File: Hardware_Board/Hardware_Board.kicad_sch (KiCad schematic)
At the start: 0 parts

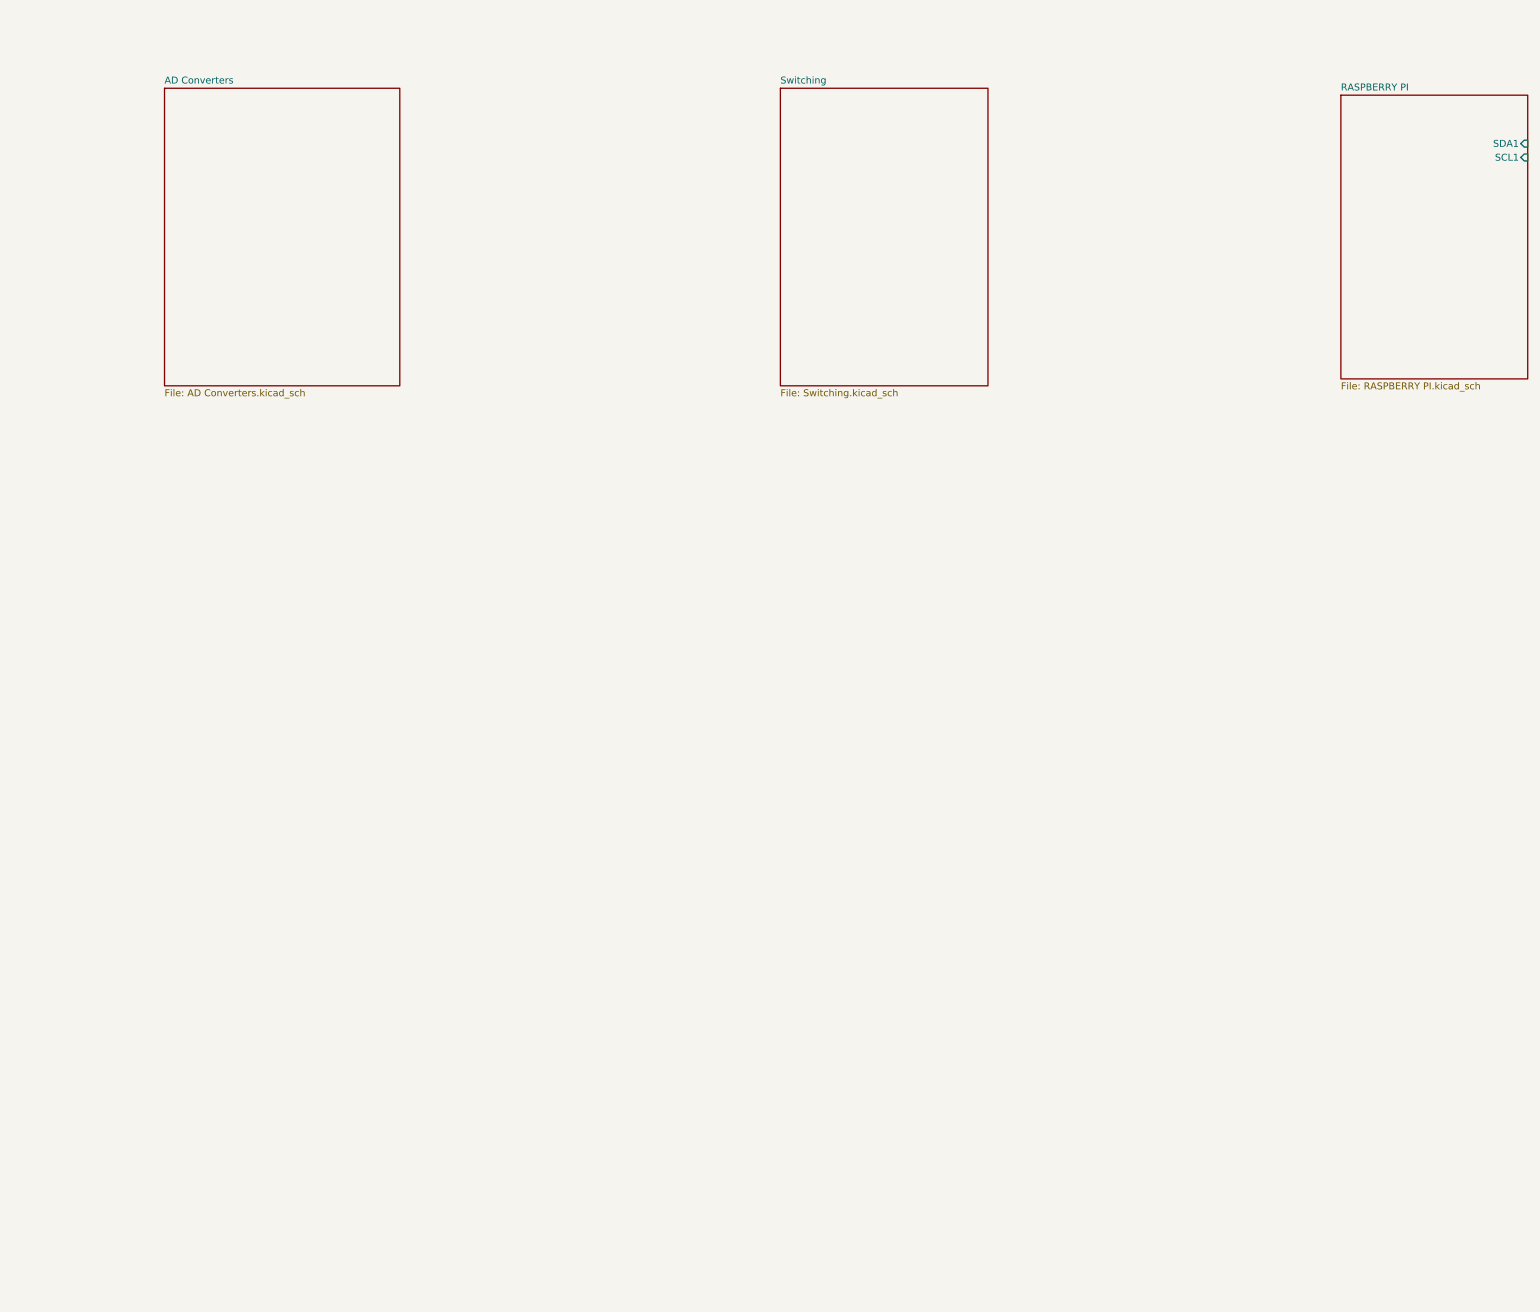
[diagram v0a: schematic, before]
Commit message: esc board updated
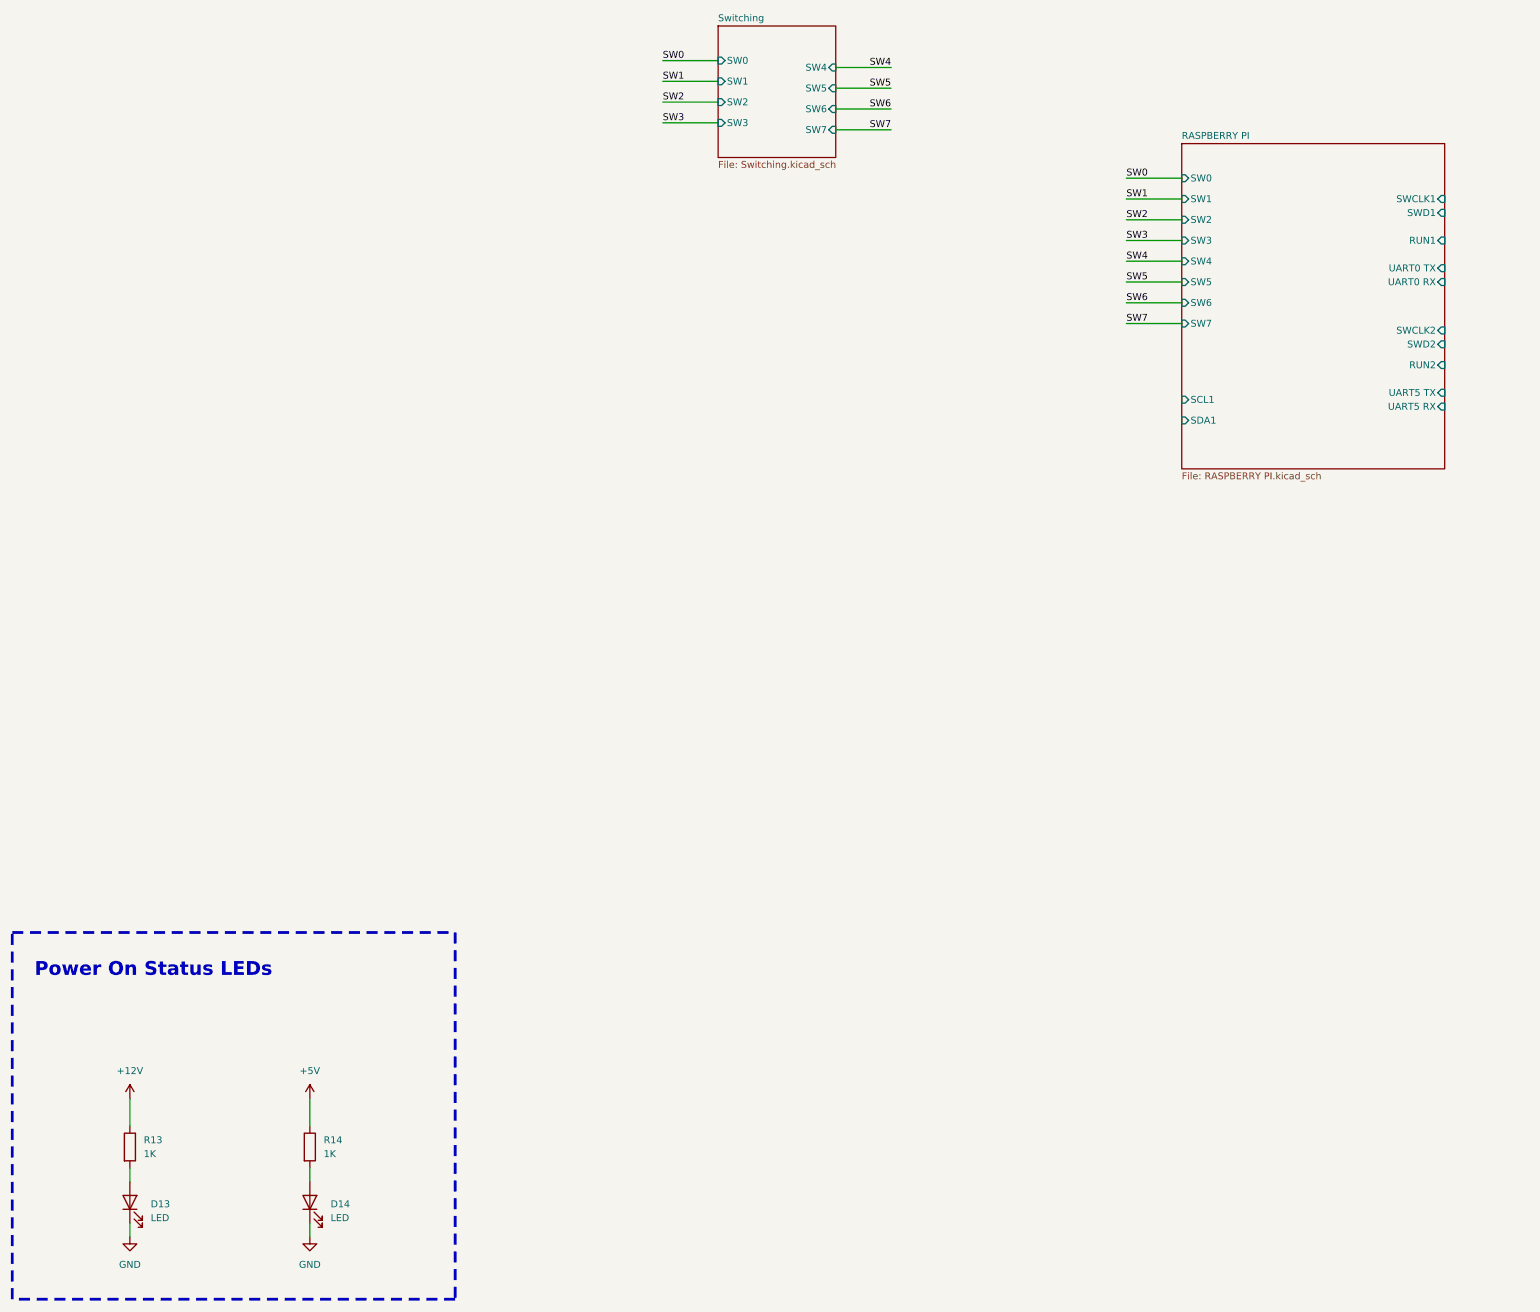
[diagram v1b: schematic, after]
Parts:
- added D13, D14: LED, symbol Device:LED
- added R13, R14: 1K, symbol Device:R
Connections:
- new net: D13.2 (A), R13.2
- new net: D14.2 (A), R14.2
- new net +12V: R13.1
- new net +5V: R14.1
- new net GND: D13.1 (K), D14.1 (K)
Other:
- removed sheet AD Converters
- sheet RASPBERRY PI ports: added RUN1, RUN2, SW0, SW1, SW2, SW3, SW4, SW5, SW6, SW7, SWCLK1, SWCLK2, SWD1, SWD2, UART0 RX, UART0 TX, UART5 RX, UART5 TX; removed none
- sheet Switching ports: added SW0, SW1, SW2, SW3, SW4, SW5, SW6, SW7; removed none
- note added: "Power On Status LEDs"
